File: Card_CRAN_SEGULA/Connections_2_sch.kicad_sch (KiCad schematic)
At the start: 40 parts, among them J4 USB4110GFA, J5 USB4110GFA, U10 CP2102N-A02-GQFN20R, U9 CP2102N-A02-GQFN20R

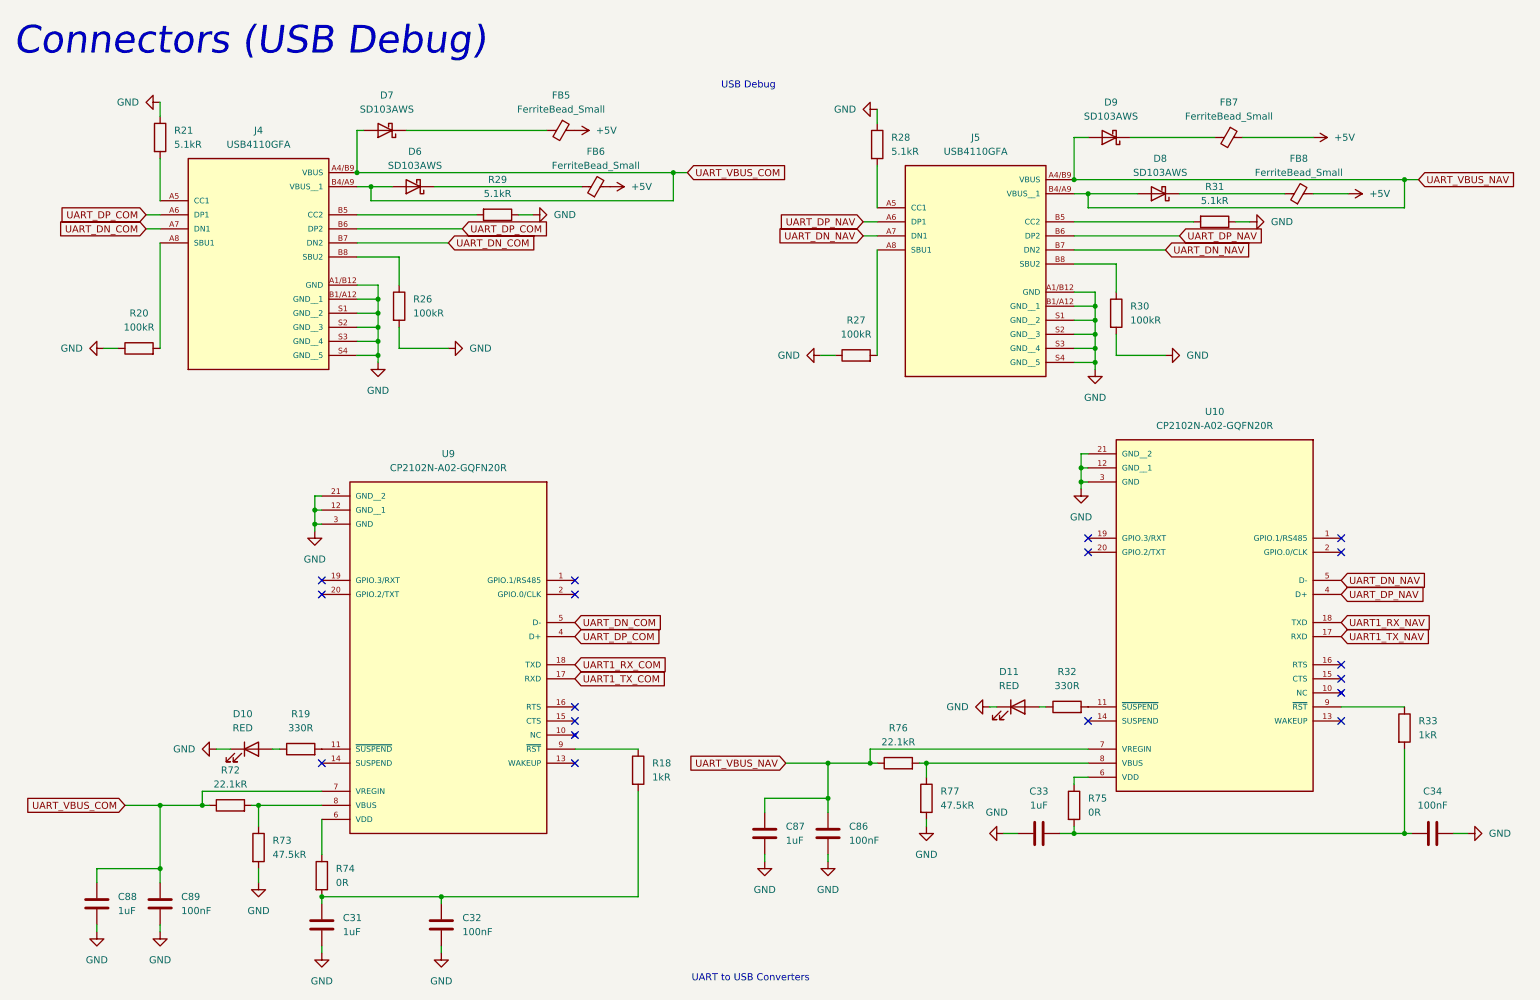
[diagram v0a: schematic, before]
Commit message: Carte presque fini avant la dernière vérification
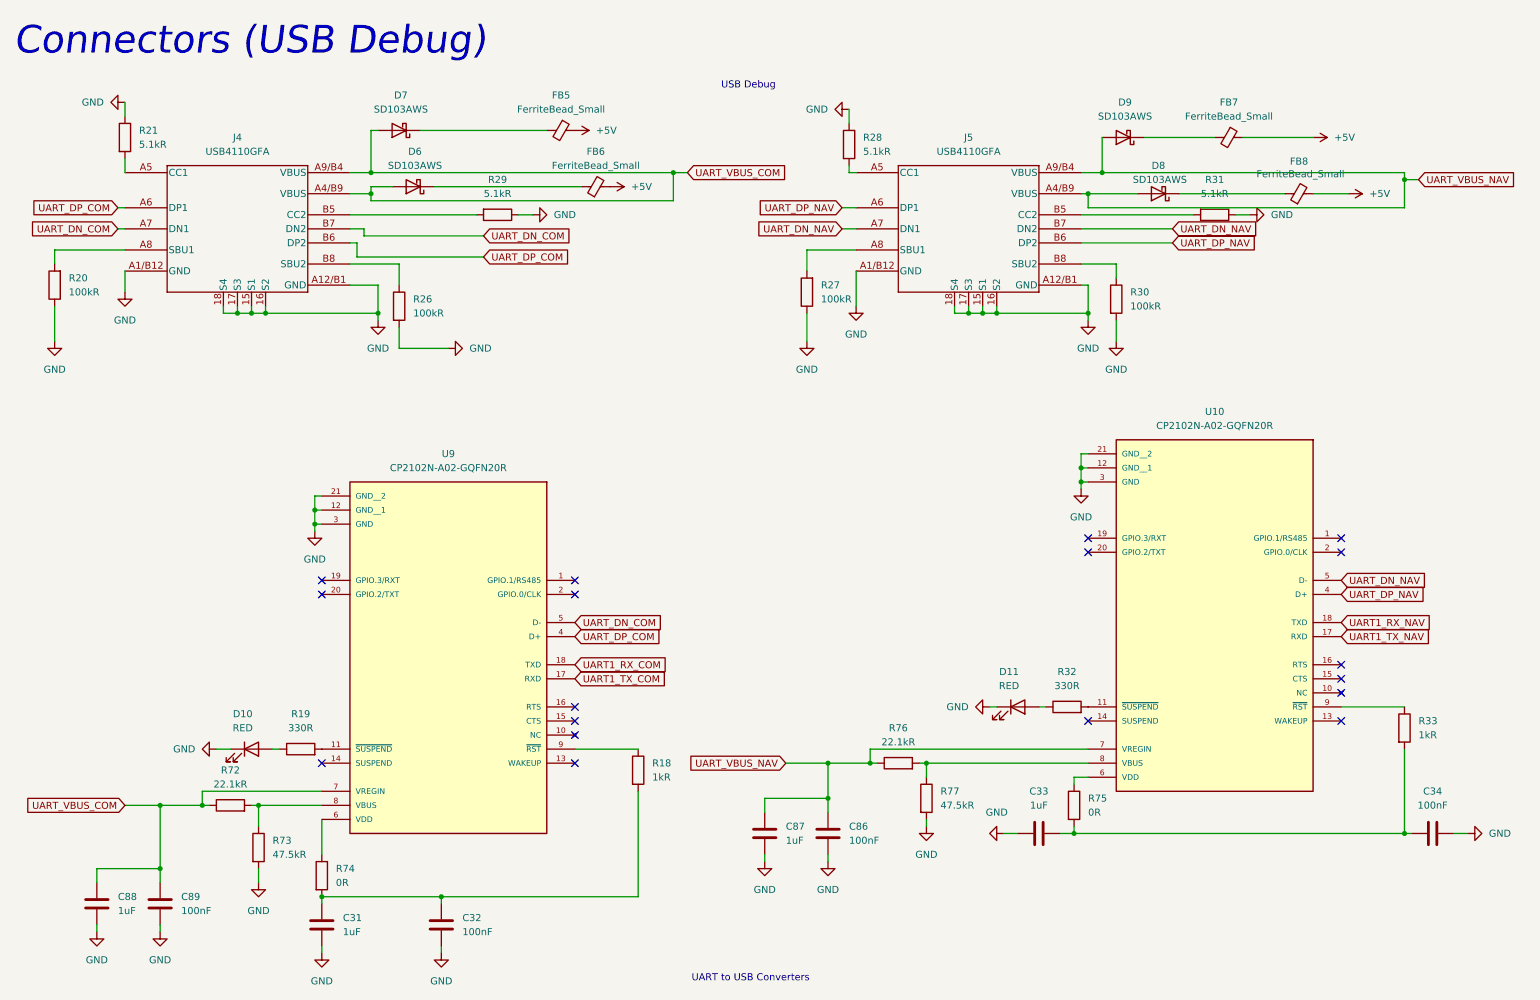
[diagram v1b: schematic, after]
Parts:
- J4, J5: footprint USB_C_USB4110GFA:GCT_USB4110GFA -> USB4110-GF-A_GCT; symbol USB_C_USB4110GFA:USB4110GFA -> USB4110GFA:USB4110-GF-A
- U10, U9: footprint UART_TO_USB_CP2102N-A02-GQFN20R:SILABS_CP2102N-A02-GQFN20R -> UART_TO_USB_CP2102N-A02-GQFN20R:QFN20_SIL
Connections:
- net GND: now also J4.15 (S1), J4.16 (S2), J4.17 (S3), J4.18 (S4), J4.A12/B1 (GND), J5.15 (S1), J5.16 (S2), J5.17 (S3), J5.18 (S4), J5.A12/B1 (GND); no longer J4.B1/A12 (GND__1), J4.S1 (GND__2), J4.S2 (GND__3), J4.S3 (GND__4), J4.S4 (GND__5), J5.B1/A12 (GND__1), J5.S1 (GND__2), J5.S2 (GND__3), J5.S3 (GND__4), J5.S4 (GND__5)
- net UART_VBUS_COM: now also J4.A9/B4 (VBUS); no longer J4.B4/A9 (VBUS__1)
- net UART_VBUS_NAV: now also J5.A9/B4 (VBUS); no longer J5.B4/A9 (VBUS__1)
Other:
- moved on the sheet: D7, D9, R20, R21, R27, R28, R30, R31
